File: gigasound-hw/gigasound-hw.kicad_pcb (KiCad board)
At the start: 2 copper layers, 115 parts, among them J1 Conn_01x05_Socket_FPC_Joycon, J2 Conn_01x05_Socket_UART, J4 USB_C_Receptacle_USB2.0_16P, J5 PIN_LED_OUT, J6 Conn_01x04_Socket_OLED, SW1 PLAY, SW2 Reset, SW4 STOP, SW5 MODE, U1 STM32F401RETx, U5 AMS1117-3.3, Y1 12MHz

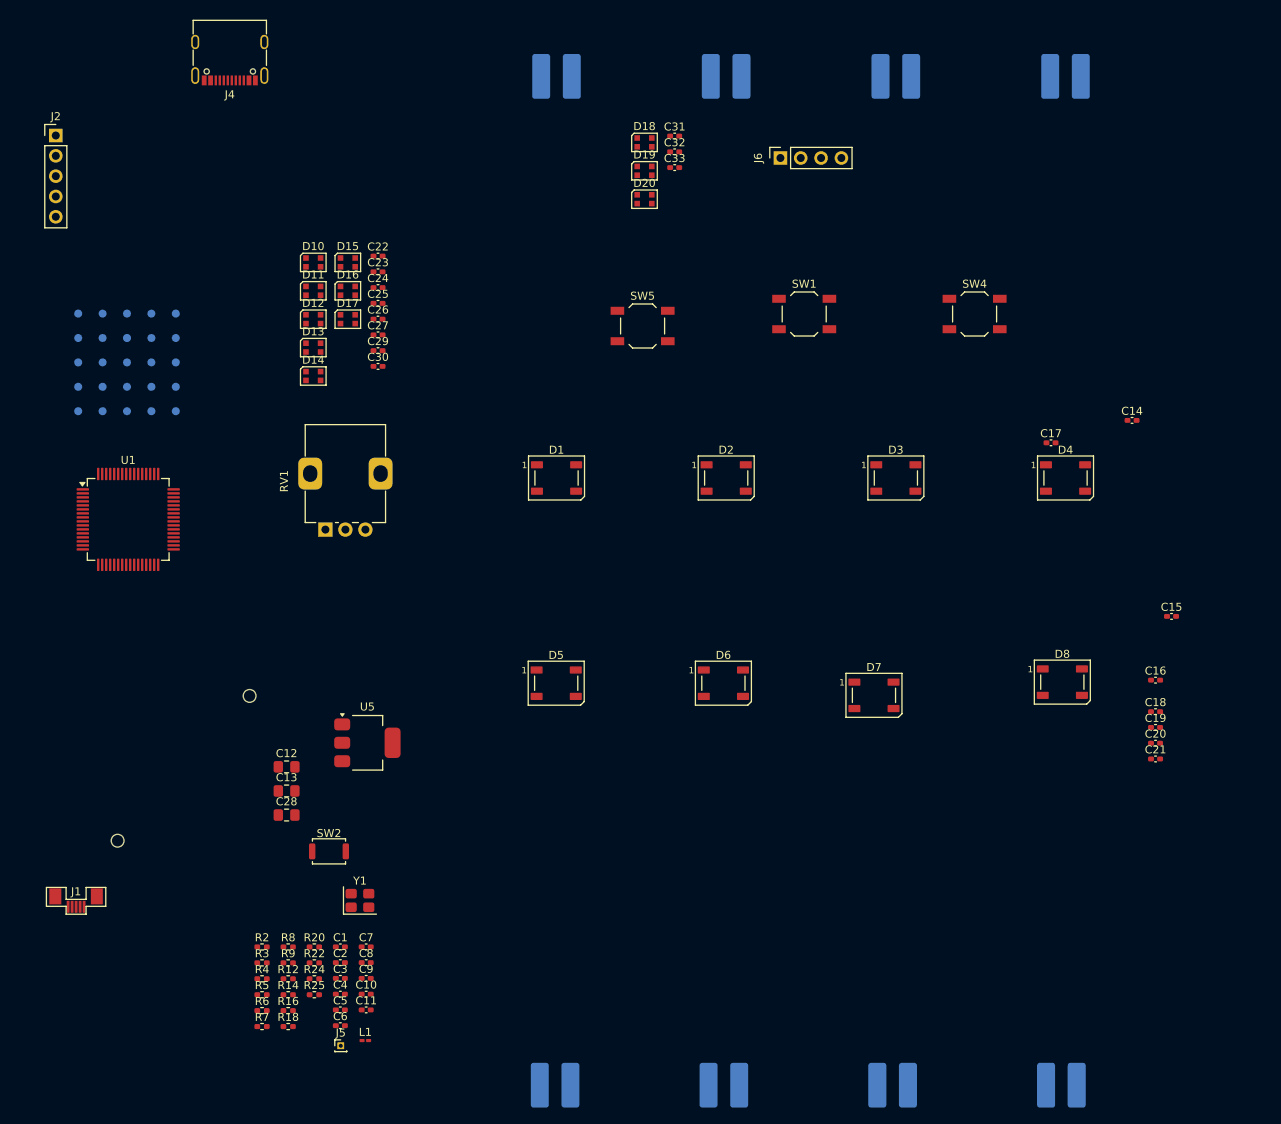
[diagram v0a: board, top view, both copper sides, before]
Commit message: hw: finish layout
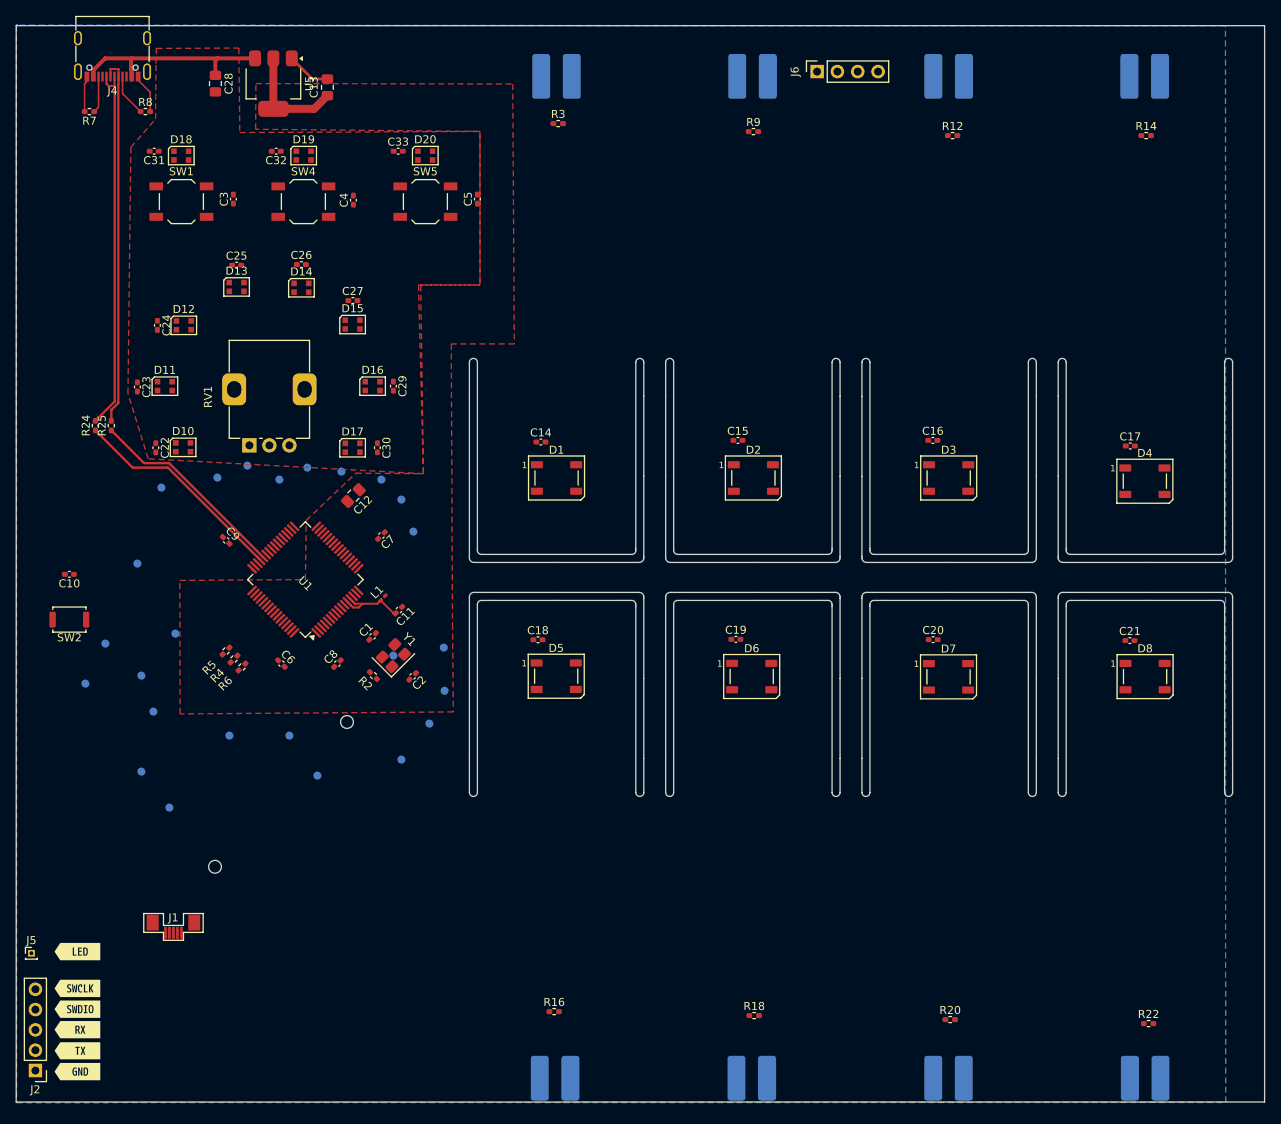
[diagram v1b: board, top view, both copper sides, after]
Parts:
- added kibuzzard-682DE080: G***, kibuzzard-682DE080, F.Cu at (55.5, 140.0)
- added kibuzzard-682DE088: G***, kibuzzard-682DE088, F.Cu at (55.5, 144.6)
- added kibuzzard-682DECE7: G***, kibuzzard-682DECE7, F.Cu at (55.5, 147.2)
- added kibuzzard-682DFB76: G***, kibuzzard-682DFB76, F.Cu at (55.5, 149.8)
- added kibuzzard-682DFB84: G***, kibuzzard-682DFB84, F.Cu at (55.5, 152.4)
- added kibuzzard-682DFB98: G***, kibuzzard-682DFB98, F.Cu at (55.5, 155.0)
- moved R14 151.8 mm to (189.1, 38.0)
- moved R12 134.2 mm to (164.9, 38.0)
- moved R9 119.1 mm to (140.0, 37.5)
- moved J2 116.9 mm to (50.2, 154.9), turned to 180 degrees
- moved R7 116.4 mm to (57.0, 35.0), turned to 180 degrees
- moved R3 111.2 mm to (115.6, 36.5)
- moved R8 105.9 mm to (64.0, 35.0)
- moved R22 104.6 mm to (189.4, 149.0)
- moved C5 102.8 mm to (105.5, 45.9), turned to 90 degrees
- moved C4 99.3 mm to (90.0, 46.1), turned to 90 degrees
- moved C3 98.3 mm to (75.0, 45.9), turned to 90 degrees
- moved C28 91.9 mm to (72.8, 31.5), turned to -90 degrees
- moved C13 88.1 mm to (86.8, 32.0), turned to 90 degrees
- moved SW4 85.1 mm to (83.8, 46.2)
- moved U5 83.2 mm to (80.0, 31.5), turned to -90 degrees
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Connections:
- net /USB_DM renamed /USB_D-
- net /USB_DP renamed /USB_D+
- U1 pad 14: /ADC_CH0 -> /ADC_CH5
- U1 pad 15: /ADC_CH1 -> /ADC_CH6
- U1 pad 16: /ADC_CH2 -> /ADC_CH7
- U1 pad 17: /ADC_CH3 -> /ADC_CH4
- U1 pad 20: /ADC_CH4 -> /ADC_CH3
- U1 pad 21: /ADC_CH5 -> /ADC_CH2
- U1 pad 22: /ADC_CH6 -> /ADC_CH1
- U1 pad 23: /ADC_CH7 -> /ADC_CH0
- Y1 pad 2: /OSC_IN -> GND
- Y1 pad 3: (no net) -> /OSC_IN
- Y1 pad 4: (no net) -> GND
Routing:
- net /USB_D-: track 0.00 -> 46.3 mm
- net /USB_D+: track 0.00 -> 46.1 mm
- net Net-(U1-PA12): track 0.00 -> 27.4 mm
- net 5V: track 0.00 -> 26.2 mm
- net Net-(U1-PA11): track 0.00 -> 25.6 mm
- net GND: track 0.00 -> 15.0 mm
- net 3.3V: track 0.00 -> 13.7 mm
- net VDDA: track 0.00 -> 9.15 mm
- net Net-(J4-CC1): track 0.00 -> 5.32 mm
- net Net-(J4-CC2): track 0.00 -> 4.60 mm
- added copper zone on F.Cu, net 3.3V
- added copper zone on F.Cu, net 5V
- added copper zone on B.Cu, net GND
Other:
- board outline added: 156.1 x 134.5 mm
